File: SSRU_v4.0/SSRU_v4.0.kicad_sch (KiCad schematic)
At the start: 71 parts, among them J2 Conn_01x24, J4 AVR-ISP-6, SW1 SW_Push, U1 SGM722, U10 TJA1051T, U2 ATmega328P-A, U3 SGM722, U4 LM2576S-5, U6 MCP2515-xST, U69 SGM722, Y1 16MHz, Y4 20MHz

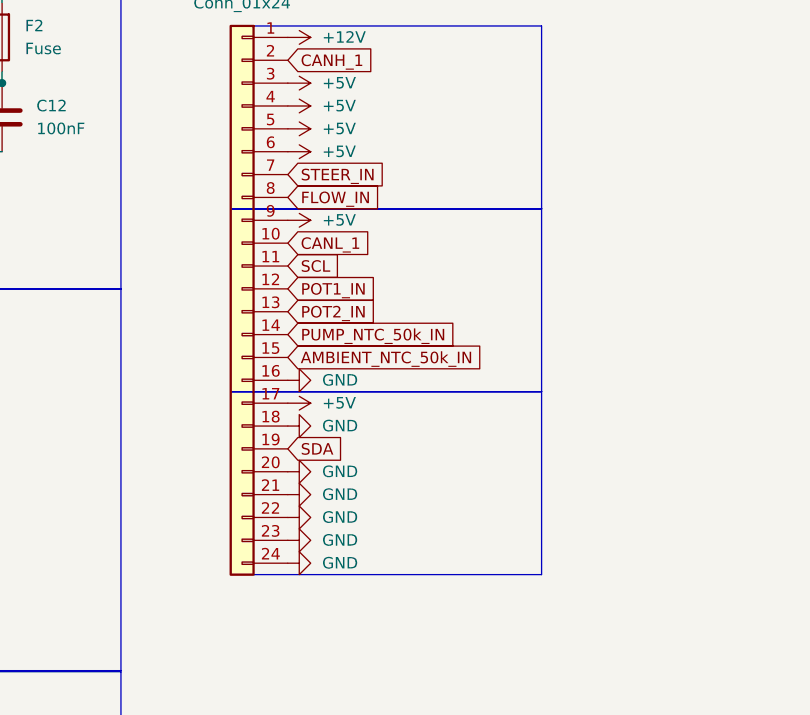
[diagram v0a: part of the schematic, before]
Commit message: gay
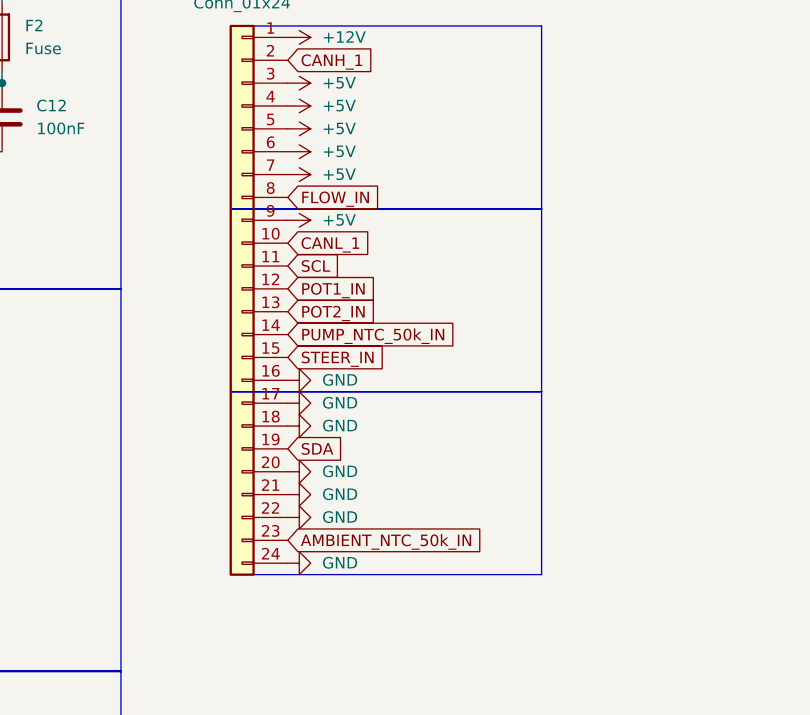
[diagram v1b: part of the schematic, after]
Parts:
- added unit 1 of U1
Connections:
- net +5V: now also J2.7 (Pin_7); no longer J2.17 (Pin_17)
- net AMBIENT_NTC_50k_IN: now also J2.23 (Pin_23), U1.3 (+); no longer J2.15 (Pin_15), U1.3 (+)
- net AMBIENT_NTC_50k_OUT: now also U1.1, U1.2 (-); no longer U1.1, U1.2 (-)
- net GND: now also J2.17 (Pin_17); no longer J2.23 (Pin_23)
- net STEER_IN: now also J2.15 (Pin_15); no longer J2.7 (Pin_7)
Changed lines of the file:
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@@
 		)
 	)
-	(global_label "AMBIENT_NTC_50k_IN"
-		(shape input)
-		(at 303.53 64.77 0)
-		(fields_autoplaced yes)
-		(effects
-			(font
-				(size 1.27 1.27)
-			)
-			(justify left)
-		)
-		(property "Intersheetrefs" "${INTERSHEET_REFS}"
-			(at 326.2304 64.77 0)
-			(effects
-				(font
-					(size 1.27 1.27)
-				)
-				(justify left)
-				(hide yes)
-			)
-		)
-	)
 	(global_label "POT2_OUT"
 		(shape output)
@@
 	(global_label "STEER_IN"
 		(shape input)
-		(at 303.53 44.45 0)
+		(at 303.53 64.77 0)
 		(fields_autoplaced yes)
 		(effects
@@
 		)
 		(property "Intersheetrefs" "${INTERSHEET_REFS}"
-			(at 315.1632 44.45 0)
+			(at 315.1632 64.77 0)
 			(effects
 				(font
@@
 		)
 	)
+	(global_label "AMBIENT_NTC_50k_IN"
+		(shape input)
+		(at 303.53 85.09 0)
+		(fields_autoplaced yes)
+		(effects
+			(font
+				(size 1.27 1.27)
+			)
+			(justify left)
+		)
+		(property "Intersheetrefs" "${INTERSHEET_REFS}"
+			(at 326.2304 85.09 0)
+			(effects
+				(font
+					(size 1.27 1.27)
+				)
+				(justify left)
+				(hide yes)
+			)
+		)
+	)
 	(global_label "CANL_1"
 		(shape input)
@@
 	)
 	(symbol
+		(lib_id "power:+5V")
+		(at 303.53 44.45 270)
+		(unit 1)
+		(exclude_from_sim no)
+		(in_bom yes)
+		(on_board yes)
+		(dnp no)
+		(property "Reference" "#PWR062"
+			(at 299.72 44.45 0)
+			(effects
+				(font
+					(size 1.27 1.27)
+				)
+				(hide yes)
+			)
+		)
+		(property "Value" "+5V"
+			(at 307.34 44.4501 90)
+			(effects
+				(font
+					(size 1.27 1.27)
+				)
+				(justify left)
+			)
+		)
+		(property "Footprint" ""
+			(at 303.53 44.45 0)
+			(effects
+				(font
+					(size 1.27 1.27)
+				)
+				(hide yes)
+			)
+		)
+		(property "Datasheet" ""
+			(at 303.53 44.45 0)
+			(effects
+				(font
+					(size 1.27 1.27)
+				)
+				(hide yes)
+			)
+		)
+		(property "Description" "Power symbol creates a global label with name \"+5V\""
+			(at 303.53 44.45 0)
+			(effects
+				(font
+					(size 1.27 1.27)
+				)
+				(hide yes)
+			)
+		)
+		(pin "1"
+		)
+		(instances
+			(project "SSRU_v4.0"
+				(path "/bee3e03c-9a5f-4c66-913e-823f7b125a2a"
+					(reference "#PWR062")
+					(unit 1)
+				)
+			)
+		)
+	)
+	(symbol
 		(lib_id "power:GND")
 		(at 303.53 80.01 90)
@@
 	(symbol
 		(lib_id "power:GND")
+		(at 303.53 69.85 90)
+		(unit 1)
+		(exclude_from_sim no)
+		(in_bom yes)
+		(on_board yes)
+		(dnp no)
+		(property "Reference" "#PWR063"
+			(at 309.88 69.85 0)
+			(effects
+				(font
+					(size 1.27 1.27)
+				)
+				(hide yes)
+			)
+		)
+		(property "Value" "GND"
+			(at 307.34 69.8499 90)
+			(effects
+				(font
+					(size 1.27 1.27)
+				)
+				(justify right)
+			)
+		)
+		(property "Footprint" ""
+			(at 303.53 69.85 0)
+			(effects
+				(font
+					(size 1.27 1.27)
+				)
+				(hide yes)
+			)
+		)
+		(property "Datasheet" ""
+			(at 303.53 69.85 0)
+			(effects
+				(font
+					(size 1.27 1.27)
+				)
+				(hide yes)
+			)
+		)
+		(property "Description" "Power symbol creates a global label with name \"GND\" , ground"
+			(at 303.53 69.85 0)
+			(effects
+				(font
+					(size 1.27 1.27)
+				)
+				(hide yes)
+			)
+		)
+		(pin "1"
+		)
+		(instances
+			(project "SSRU_v4.0"
+				(path "/bee3e03c-9a5f-4c66-913e-823f7b125a2a"
+					(reference "#PWR063")
+					(unit 1)
+				)
+			)
+		)
+	)
+	(symbol
+		(lib_id "power:GND")
 		(at 135.89 189.23 0)
 		(unit 1)
@@
 	)
 	(symbol
-		(lib_id "power:GND")
-		(at 303.53 85.09 90)
-		(mirror x)
-		(unit 1)
-		(exclude_from_sim no)
-		(in_bom yes)
-		(on_board yes)
-		(dnp no)
-		(fields_autoplaced yes)
-		(property "Reference" "#PWR062"
-			(at 309.88 85.09 0)
-			(effects
-				(font
-					(size 1.27 1.27)
-				)
-				(hide yes)
-			)
-		)
-		(property "Value" "GND"
-			(at 307.34 85.0899 90)
-			(effects
-				(font
-					(size 1.27 1.27)
-				)
-				(justify right)
-			)
-		)
-		(property "Footprint" ""
-			(at 303.53 85.09 0)
-			(effects
-				(font
-					(size 1.27 1.27)
-				)
-				(hide yes)
-			)
-		)
-		(property "Datasheet" ""
-			(at 303.53 85.09 0)
-			(effects
-				(font
-					(size 1.27 1.27)
-				)
-				(hide yes)
-			)
-		)
-		(property "Description" "Power symbol creates a global label with name \"GND\" , ground"
-			(at 303.53 85.09 0)
-			(effects
-				(font
-					(size 1.27 1.27)
-				)
-				(hide yes)
-			)
-		)
-		(pin "1"
-		)
-		(instances
-			(project "SSRU_v4.0"
-				(path "/bee3e03c-9a5f-4c66-913e-823f7b125a2a"
-					(reference "#PWR062")
-					(unit 1)
-				)
-			)
-		)
-	)
-	(symbol
 		(lib_id "power:+5V")
 		(at 379.73 179.07 0)
@@
 					(unit 1)
 				)
-			)
-		)
-	)
-	(symbol
-		(lib_id "power:+5V")
-		(at 303.53 69.85 270)
-		(unit 1)
-		(exclude_from_sim no)
-		(in_bom yes)
-		(on_board yes)
-		(dnp no)
-		(property "Reference" "#PWR089"
-			(at 299.72 69.85 0)
-			(effects
-				(font
-					(size 1.27 1.27)
-				)
-				(hide yes)
-			)
-		)
-		(property "Value" "+5V"
-			(at 307.34 69.8501 90)
-			(effects
-				(font
-					(size 1.27 1.27)
-				)
-				(justify left)
-			)
-		)
-		(property "Footprint" ""
-			(at 303.53 69.85 0)
-			(effects
-				(font
-					(size 1.27 1.27)
-				)
-				(hide yes)
-			)
-		)
-		(property "Datasheet" ""
-			(at 303.53 69.85 0)
-			(effects
-				(font
-					(size 1.27 1.27)
-				)
-				(hide yes)
-			)
-		)
-		(property "Description" "Power symbol creates a global label with name \"+5V\""
-			(at 303.53 69.85 0)
-			(effects
-				(font
-					(size 1.27 1.27)
-				)
-				(hide yes)
-			)
-		)
-		(pin "1"
-		)
-		(instances
-			(project "SSRU_v3.2"
-				(path "/bee3e03c-9a5f-4c66-913e-823f7b125a2a"
-					(reference "#PWR089")
-					(unit 1)
-				)
